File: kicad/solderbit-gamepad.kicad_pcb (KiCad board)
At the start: 2 copper layers, 114 x 49.3 mm, 38 parts, among them CN1 SMTSOM310BTR, CN2 SMTSOM310BTR, CN3 SMTSOM310BTR, CN4 SMTSOM310BTR, CN5 SMTSOM310BTR, J2 S2B-PH-SM4-TB(LF)(SN), Q1 DMG2045U, SW1 MST22D18G2 125, U1 74HC165D,653, U2 NCP114ASN330T1G

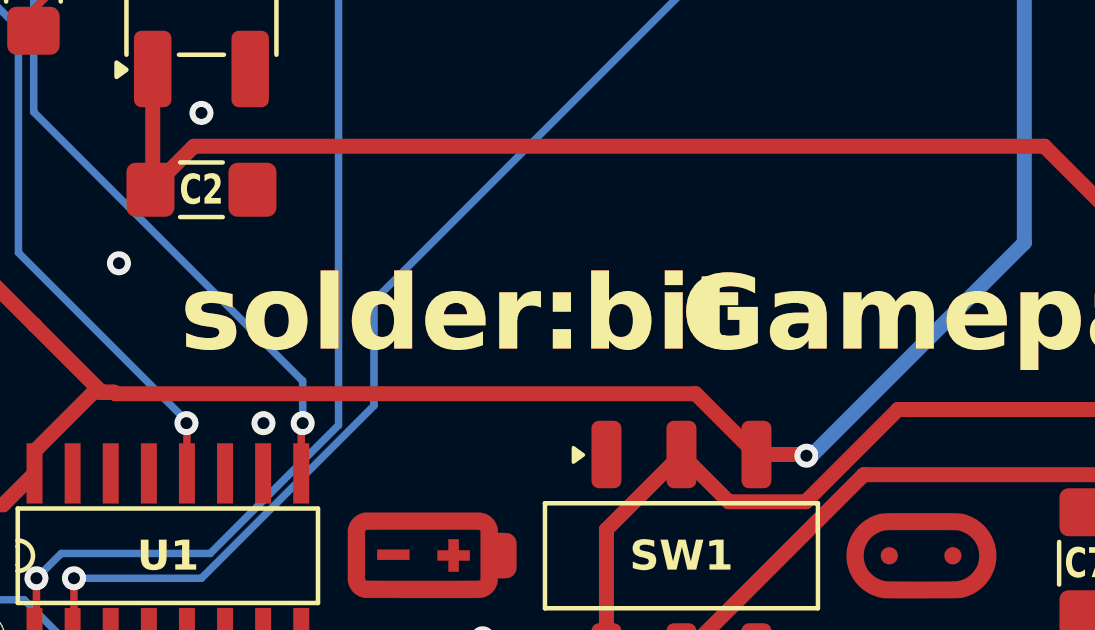
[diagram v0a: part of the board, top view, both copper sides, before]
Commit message: Cleanup, and add new images
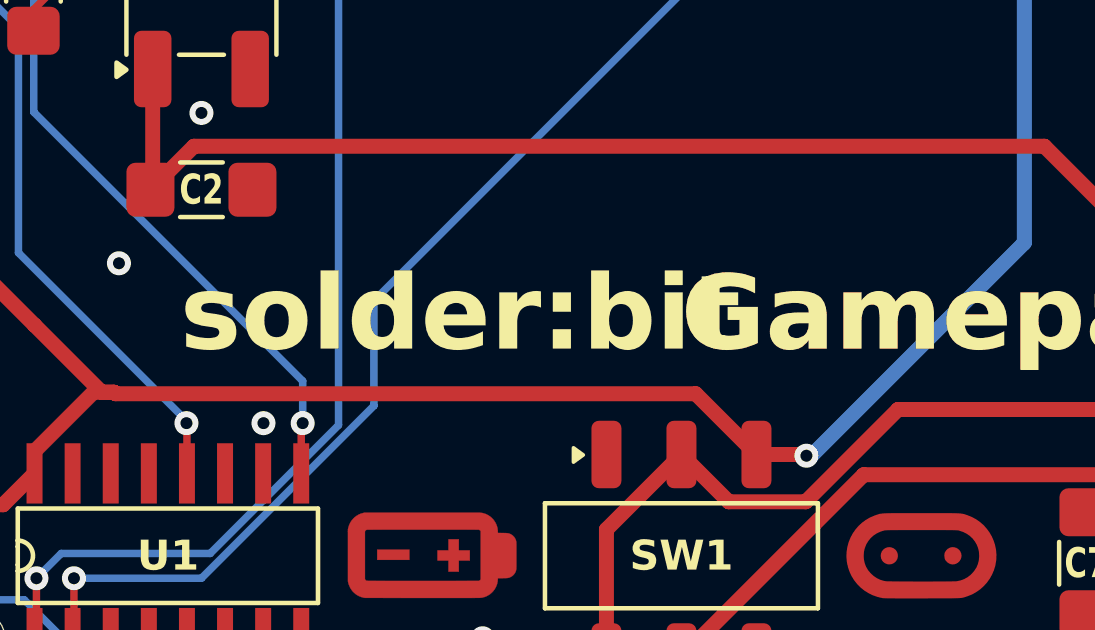
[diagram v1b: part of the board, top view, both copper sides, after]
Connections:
- net BTN_DOWN renamed /BTN_DOWN
- net BTN_LEFT renamed /BTN_LEFT
- net BTN_L_BUMP renamed /BTN_L_BUMP
- net BTN_RIGHT renamed /BTN_RIGHT
- net BTN_R_BUMP renamed /BTN_R_BUMP
- net BTN_UP renamed /BTN_UP
- net BTN_X renamed /BTN_X
- net BTN_Y renamed /BTN_Y
- net CLK renamed /CLK
- net PL/DATA renamed /PL/DATA
- net SER renamed /SER
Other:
- board text added: "placeholder"
- board text removed: "placeholder (delete me)"
